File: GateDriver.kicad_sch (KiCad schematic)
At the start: 11 parts, among them U4 IR2110

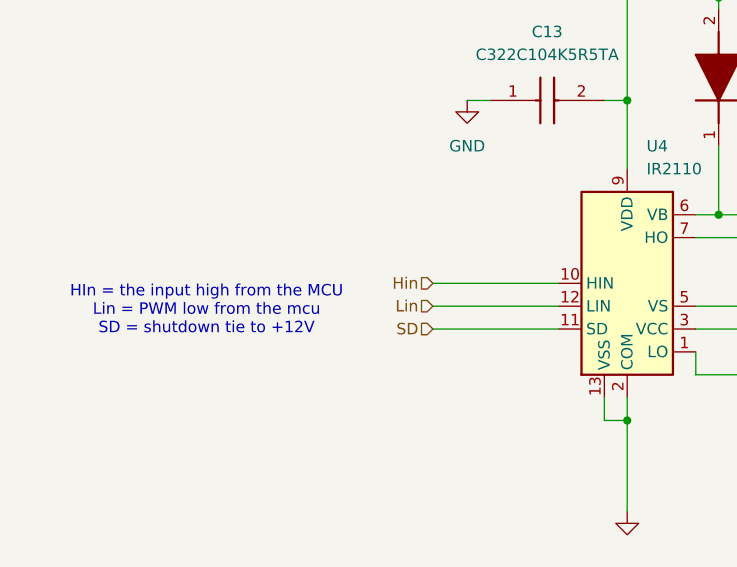
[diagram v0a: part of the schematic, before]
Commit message: Autosave
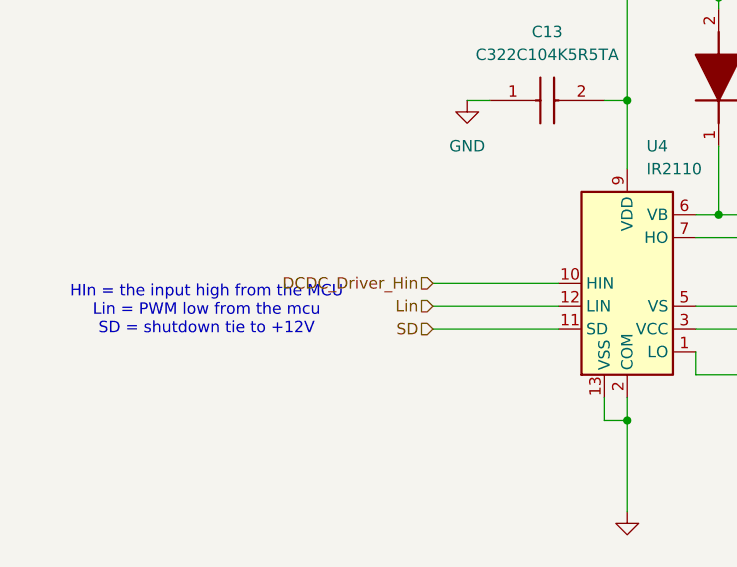
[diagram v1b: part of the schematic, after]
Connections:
- net Hin renamed DCDC_Driver_Hin
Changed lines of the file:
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@@
 		)
 	)
-	(hierarchical_label "Hin"
+	(hierarchical_label "DCDC_Driver_Hin"
 		(shape input)
 		(at 60.96 58.42 180)

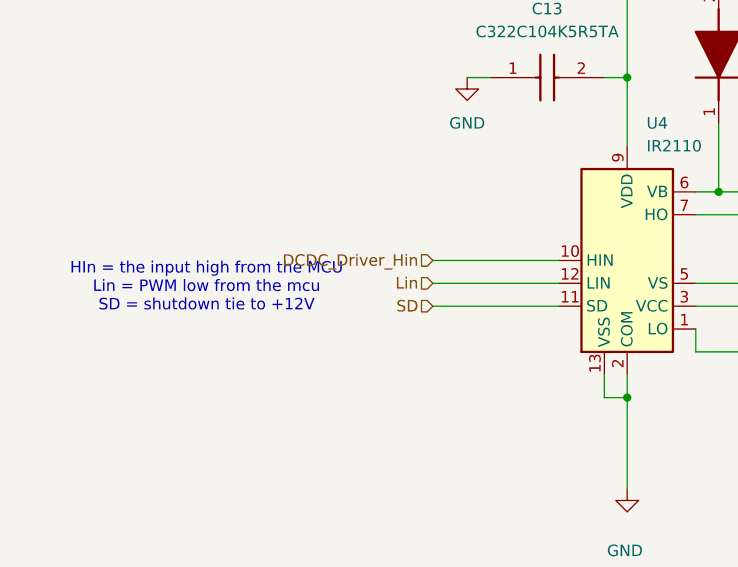
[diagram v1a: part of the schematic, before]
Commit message: Autosave
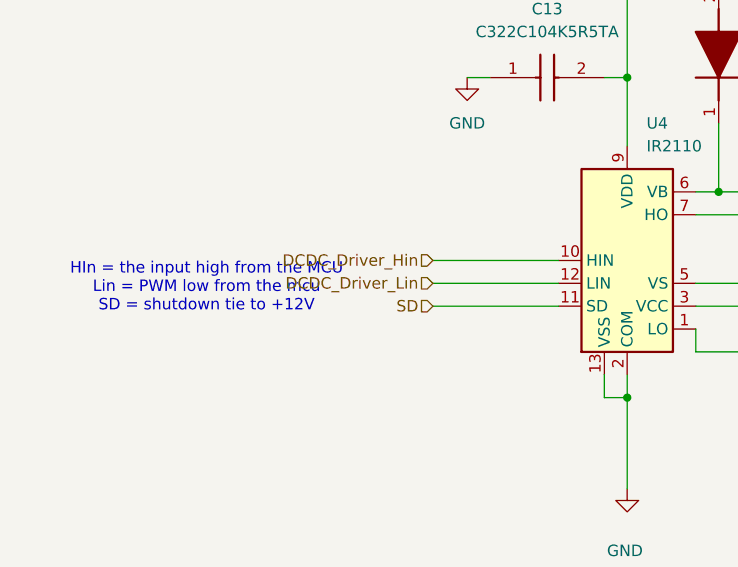
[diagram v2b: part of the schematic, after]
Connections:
- net Lin renamed DCDC_Driver_Lin
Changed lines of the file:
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@@
 		)
 	)
-	(hierarchical_label "Lin"
+	(hierarchical_label "DCDC_Driver_Lin"
 		(shape input)
 		(at 60.96 60.96 180)

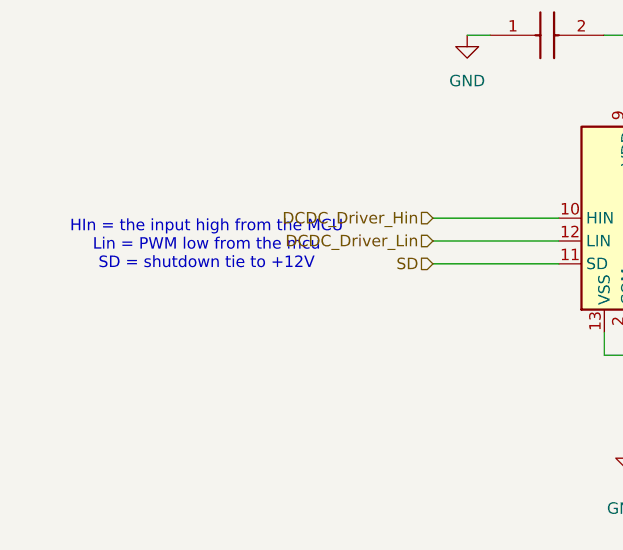
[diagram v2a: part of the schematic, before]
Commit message: Autosave
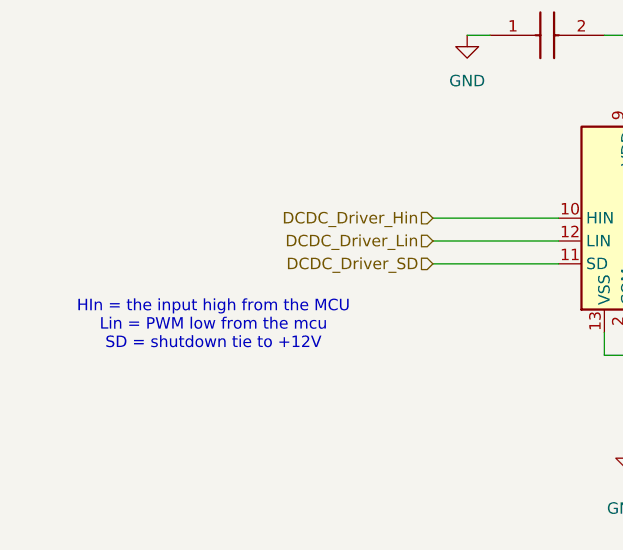
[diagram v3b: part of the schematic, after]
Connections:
- net SD renamed DCDC_Driver_SD
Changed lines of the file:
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@@
 	(text "HIn = the input high from the MCU\nLin = PWM low from the mcu\nSD = shutdown tie to +12V"
 		(exclude_from_sim no)
-		(at 35.814 61.468 0)
+		(at 36.576 70.358 0)
 		(effects
 			(font
@@
 		)
 	)
-	(hierarchical_label "SD"
+	(hierarchical_label "DCDC_Driver_SD"
 		(shape input)
 		(at 60.96 63.5 180)

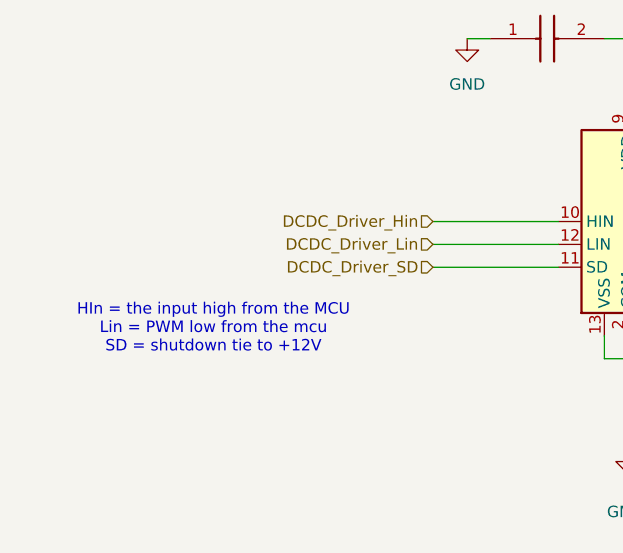
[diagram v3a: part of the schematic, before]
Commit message: SCH Save: 2 files changed GateDriver.kicad_sch 0/0/4 inverter.kicad_sch 28/0/10
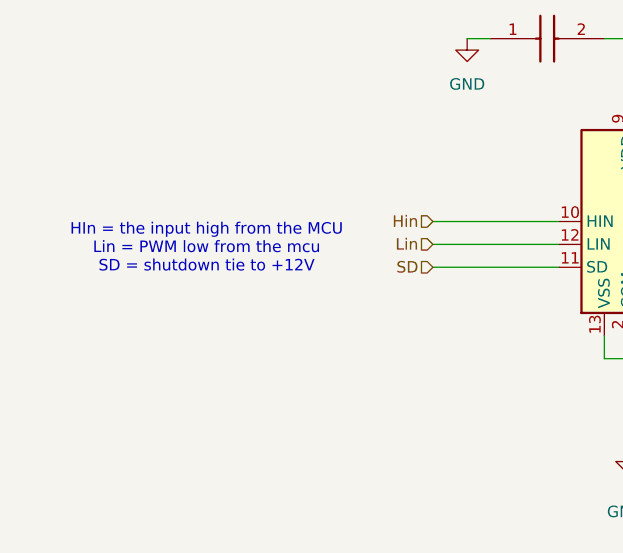
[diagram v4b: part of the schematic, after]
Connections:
- net DCDC_Driver_Hin renamed Hin
- net DCDC_Driver_Lin renamed Lin
- net DCDC_Driver_SD renamed SD
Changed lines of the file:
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@@
 	(text "HIn = the input high from the MCU\nLin = PWM low from the mcu\nSD = shutdown tie to +12V"
 		(exclude_from_sim no)
-		(at 36.576 70.358 0)
+		(at 35.814 61.468 0)
 		(effects
 			(font
@@
 		)
 	)
-	(hierarchical_label "DCDC_Driver_Lin"
+	(hierarchical_label "Lin"
 		(shape input)
 		(at 60.96 60.96 180)
@@
 		)
 	)
-	(hierarchical_label "DCDC_Driver_SD"
+	(hierarchical_label "SD"
 		(shape input)
 		(at 60.96 63.5 180)
@@
 		)
 	)
-	(hierarchical_label "DCDC_Driver_Hin"
+	(hierarchical_label "Hin"
 		(shape input)
 		(at 60.96 58.42 180)
